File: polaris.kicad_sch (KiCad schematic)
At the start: 17 parts, among them J101 XT60-M, J102 Screw_Terminal_01x02, J103 Screw_Terminal_01x02, J104 Screw_Terminal_01x02, J105 Screw_Terminal_01x02, J106 Screw_Terminal_01x02, J107 Screw_Terminal_01x02, J108 Screw_Terminal_01x03, J109 Screw_Terminal_01x03, J110 Screw_Terminal_01x03, J111 Screw_Terminal_01x03, J112 Conn_01x04, J113 Conn_01x04

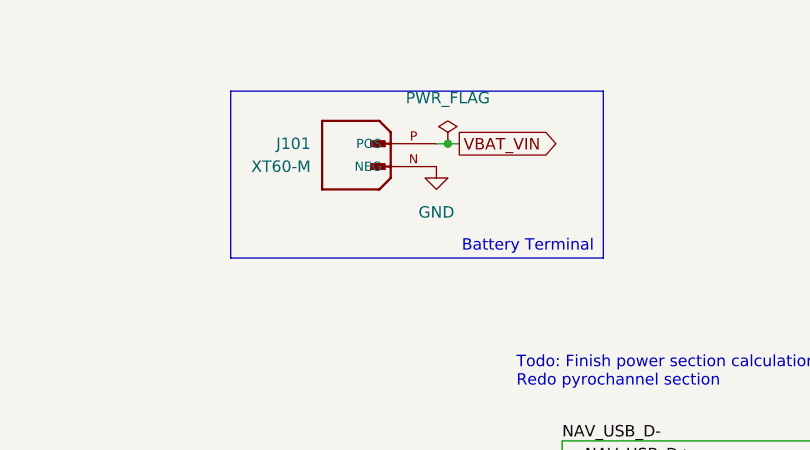
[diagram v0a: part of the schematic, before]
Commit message: Add files via upload
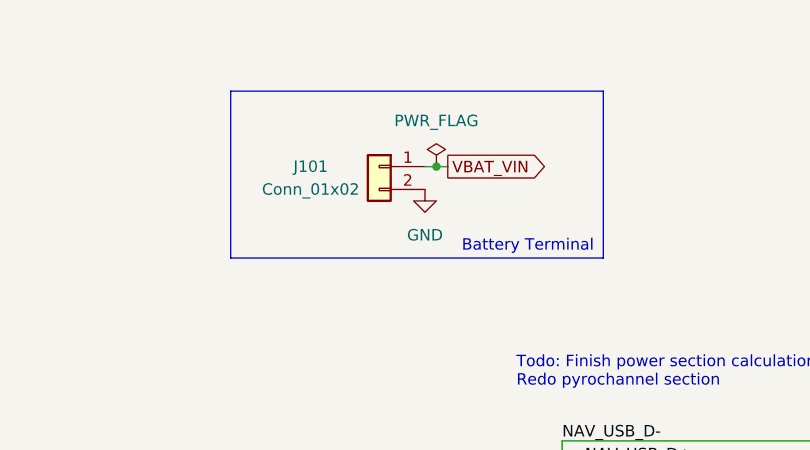
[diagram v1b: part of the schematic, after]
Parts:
- removed J101: XT60-M, Connector_AMASS:AMASS_XT60-M_1x02_P7.20mm_Vertical, symbol xt60:XT60-M
- added J101: Conn_01x02, Connector_AMASS:AMASS_XT60-M_1x02_P7.20mm_Vertical, symbol Connector_Generic:Conn_01x02
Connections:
- net GND: now also J101.2 (Pin_2)
- net VBAT_VIN: now also J101.1 (Pin_1)
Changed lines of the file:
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@@
 	)
 	(junction
-		(at 80.01 35.56)
+		(at 78.74 38.1)
 		(diameter 0)
 		(color 0 0 0 0)
@@
 	(wire
 		(pts
-			(xy 80.01 35.56) (xy 81.28 35.56)
+			(xy 78.74 38.1) (xy 80.01 38.1)
 		)
 		(stroke
@@
 	(wire
 		(pts
-			(xy 78.74 35.56) (xy 80.01 35.56)
+			(xy 77.47 38.1) (xy 78.74 38.1)
 		)
 		(stroke
@@
 	(global_label "VBAT_VIN"
 		(shape output)
-		(at 81.28 35.56 0)
+		(at 80.01 38.1 0)
 		(fields_autoplaced yes)
 		(effects
@@
 		)
 		(property "Intersheetrefs" "${INTERSHEET_REFS}"
-			(at 92.6715 35.56 0)
+			(at 91.4015 38.1 0)
 			(hide yes)
 			(show_name no)
@@
 	)
 	(symbol
-		(lib_id "xt60:XT60-M")
-		(at 73.66 38.1 0)
-		(mirror y)
-		(unit 1)
-		(body_style 1)
-		(exclude_from_sim no)
-		(in_bom yes)
-		(on_board yes)
-		(in_pos_files yes)
-		(dnp no)
-		(fields_autoplaced yes)
-		(property "Reference" "J101"
-			(at 64.77 35.5599 0)
-			(show_name no)
-			(do_not_autoplace no)
-			(effects
-				(font
-					(size 1.27 1.27)
-				)
-				(justify left)
-			)
-		)
-		(property "Value" "XT60-M"
-			(at 64.77 38.0999 0)
-			(show_name no)
-			(do_not_autoplace no)
-			(effects
-				(font
-					(size 1.27 1.27)
-				)
-				(justify left)
-			)
-		)
-		(property "Footprint" "Connector_AMASS:AMASS_XT60-M_1x02_P7.20mm_Vertical"
-			(at 73.66 38.1 0)
-			(hide yes)
-			(show_name no)
-			(do_not_autoplace no)
-			(effects
-				(font
-					(size 1.27 1.27)
-				)
-				(justify bottom)
-			)
-		)
-		(property "Datasheet" ""
-			(at 73.66 38.1 0)
-			(hide yes)
-			(show_name no)
-			(do_not_autoplace no)
-			(effects
-				(font
-					(size 1.27 1.27)
-				)
-			)
-		)
-		(property "Description" ""
-			(at 73.66 38.1 0)
-			(hide yes)
-			(show_name no)
-			(do_not_autoplace no)
-			(effects
-				(font
-					(size 1.27 1.27)
-				)
-			)
-		)
-		(property "MF" "AMASS"
-			(at 73.66 38.1 0)
-			(hide yes)
-			(show_name no)
-			(do_not_autoplace no)
-			(effects
-				(font
-					(size 1.27 1.27)
-				)
-				(justify bottom)
-			)
-		)
-		(property "MAXIMUM_PACKAGE_HEIGHT" "16.00 mm"
-			(at 73.66 38.1 0)
-			(hide yes)
-			(show_name no)
-			(do_not_autoplace no)
-			(effects
-				(font
-					(size 1.27 1.27)
-				)
-				(justify bottom)
-			)
-		)
-		(property "Package" "Package"
-			(at 73.66 38.1 0)
-			(hide yes)
-			(show_name no)
-			(do_not_autoplace no)
-			(effects
-				(font
-					(size 1.27 1.27)
-				)
-				(justify bottom)
-			)
-		)
-		(property "Price" "None"
-			(at 73.66 38.1 0)
-			(hide yes)
-			(show_name no)
-			(do_not_autoplace no)
-			(effects
-				(font
-					(size 1.27 1.27)
-				)
-				(justify bottom)
-			)
-		)
-		(property "Check_prices" "https://www.snapeda.com/parts/XT60-M/AMASS/view-part/?ref=eda"
-			(at 73.66 38.1 0)
-			(hide yes)
-			(show_name no)
-			(do_not_autoplace no)
-			(effects
-				(font
-					(size 1.27 1.27)
-				)
-				(justify bottom)
-			)
-		)
-		(property "STANDARD" "IPC 7351B"
-			(at 73.66 38.1 0)
-			(hide yes)
-			(show_name no)
-			(do_not_autoplace no)
-			(effects
-				(font
-					(size 1.27 1.27)
-				)
-				(justify bottom)
-			)
-		)
-		(property "PARTREV" "V1.2"
-			(at 73.66 38.1 0)
-			(hide yes)
-			(show_name no)
-			(do_not_autoplace no)
-			(effects
-				(font
-					(size 1.27 1.27)
-				)
-				(justify bottom)
-			)
-		)
-		(property "SnapEDA_Link" "https://www.snapeda.com/parts/XT60-M/AMASS/view-part/?ref=snap"
-			(at 73.66 38.1 0)
-			(hide yes)
-			(show_name no)
-			(do_not_autoplace no)
-			(effects
-				(font
-					(size 1.27 1.27)
-				)
-				(justify bottom)
-			)
-		)
-		(property "MP" "XT60-M"
-			(at 73.66 38.1 0)
-			(hide yes)
-			(show_name no)
-			(do_not_autoplace no)
-			(effects
-				(font
-					(size 1.27 1.27)
-				)
-				(justify bottom)
-			)
-		)
-		(property "Description_1" "Plug; DC supply; XT60; male; PIN: 2; for cable; soldered; 30A; 500V"
-			(at 73.66 38.1 0)
-			(hide yes)
-			(show_name no)
-			(do_not_autoplace no)
-			(effects
-				(font
-					(size 1.27 1.27)
-				)
-				(justify bottom)
-			)
-		)
-		(property "Availability" "In Stock"
-			(at 73.66 38.1 0)
-			(hide yes)
-			(show_name no)
-			(do_not_autoplace no)
-			(effects
-				(font
-					(size 1.27 1.27)
-				)
-				(justify bottom)
-			)
-		)
-		(property "MANUFACTURER" "AMASS"
-			(at 73.66 38.1 0)
-			(hide yes)
-			(show_name no)
-			(do_not_autoplace no)
-			(effects
-				(font
-					(size 1.27 1.27)
-				)
-				(justify bottom)
-			)
-		)
-		(pin "N"
-		)
-		(pin "P"
-		)
-		(instances
-			(project "polaris"
-				(path "/cfb90e19-9fbe-47a1-a5ac-df522853d1d0"
-					(reference "J101")
-					(unit 1)
-				)
-			)
-		)
-	)
-	(symbol
 		(lib_id "Connector:Screw_Terminal_01x02")
 		(at 254 139.7 0)
@@
 	(symbol
 		(lib_id "power:GND")
-		(at 78.74 38.1 0)
+		(at 77.47 40.64 0)
 		(unit 1)
 		(body_style 1)
@@
 		(fields_autoplaced yes)
 		(property "Reference" "#PWR0101"
-			(at 78.74 44.45 0)
+			(at 77.47 46.99 0)
 			(hide yes)
 			(show_name no)
@@
 		)
 		(property "Value" "GND"
-			(at 78.74 43.18 0)
+			(at 77.47 45.72 0)
 			(show_name no)
 			(do_not_autoplace no)
@@
 		)
 		(property "Footprint" ""
-			(at 78.74 38.1 0)
+			(at 77.47 40.64 0)
 			(hide yes)
 			(show_name no)
@@
 		)
 		(property "Datasheet" ""
-			(at 78.74 38.1 0)
+			(at 77.47 40.64 0)
 			(hide yes)
 			(show_name no)
@@
 		)
 		(property "Description" "Power symbol creates a global label with name \"GND\" , ground"
-			(at 78.74 38.1 0)
+			(at 77.47 40.64 0)
 			(hide yes)
 			(show_name no)
@@
 	(symbol
 		(lib_id "power:PWR_FLAG")
-		(at 80.01 35.56 0)
+		(at 78.74 38.1 0)
 		(unit 1)
 		(body_style 1)
@@
 		(fields_autoplaced yes)
 		(property "Reference" "#FLG0101"
-			(at 80.01 33.655 0)
+			(at 78.74 36.195 0)
 			(hide yes)
 			(show_name no)
@@
 		)
 		(property "Value" "PWR_FLAG"
-			(at 80.01 30.48 0)
+			(at 78.74 33.02 0)
 			(show_name no)
 			(do_not_autoplace no)
@@
 		)
 		(property "Footprint" ""
-			(at 80.01 35.56 0)
+			(at 78.74 38.1 0)
 			(hide yes)
 			(show_name no)
@@
 		)
 		(property "Datasheet" ""
-			(at 80.01 35.56 0)
+			(at 78.74 38.1 0)
 			(hide yes)
 			(show_name no)
@@
 		)
 		(property "Description" "Special symbol for telling ERC where power comes from"
-			(at 80.01 35.56 0)
+			(at 78.74 38.1 0)
 			(hide yes)
 			(show_name no)
@@
 					(unit 1)
 				)
+			)
+		)
+	)
+	(symbol
+		(lib_id "Connector_Generic:Conn_01x02")
+		(at 72.39 38.1 0)
+		(mirror y)
+		(unit 1)
+		(body_style 1)
+		(exclude_from_sim no)
+		(in_bom yes)
+		(on_board yes)
+		(in_pos_files yes)
+		(dnp no)
+		(property "Reference" "J101"
+			(at 64.77 38.1 0)
+			(show_name no)
+			(do_not_autoplace no)
+			(effects
+				(font
+					(size 1.27 1.27)
+				)
+			)
+		)
+		(property "Value" "Conn_01x02"
+			(at 64.77 40.64 0)
+			(show_name no)
+			(do_not_autoplace no)
+			(effects
+				(font
+					(size 1.27 1.27)
+				)
+			)
+		)
+		(property "Footprint" "Connector_AMASS:AMASS_XT60-M_1x02_P7.20mm_Vertical"
+			(at 72.39 38.1 0)
+			(hide yes)
+			(show_name no)
+			(do_not_autoplace no)
+			(effects
+				(font
+					(size 1.27 1.27)
+				)
+			)
+		)
+		(property "Datasheet" ""
+			(at 72.39 38.1 0)
+			(hide yes)
+			(show_name no)
+			(do_not_autoplace no)
+			(effects
+				(font
+					(size 1.27 1.27)
+				)
+			)
+		)
+		(property "Description" "Generic connector, single row, 01x02, script generated (kicad-library-utils/schlib/autogen/connector/)"
+			(at 72.39 38.1 0)
+			(hide yes)
+			(show_name no)
+			(do_not_autoplace no)
+			(effects
+				(font
+					(size 1.27 1.27)
+				)
+			)
+		)
+		(pin "1"
+		)
+		(pin "2"
+		)
+		(instances
+			(project "polaris"
+				(path "/cfb90e19-9fbe-47a1-a5ac-df522853d1d0"
+					(reference "J101")
+					(unit 1)
+				)
